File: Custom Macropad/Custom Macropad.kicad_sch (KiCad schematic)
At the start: 25 parts, among them SW1 RotaryEncoder_Switch, SW10 SW_Push, SW11 SW_Push, SW12 SW_Push, SW17 RotaryEncoder_Switch, SW2 SW_Push, SW3 SW_Push, SW5 SW_Push, SW6 SW_Push, SW7 SW_Push, SW8 SW_Push, SW9 SW_Push, U1 MOUDLE-SEEEDUINO-XIAO

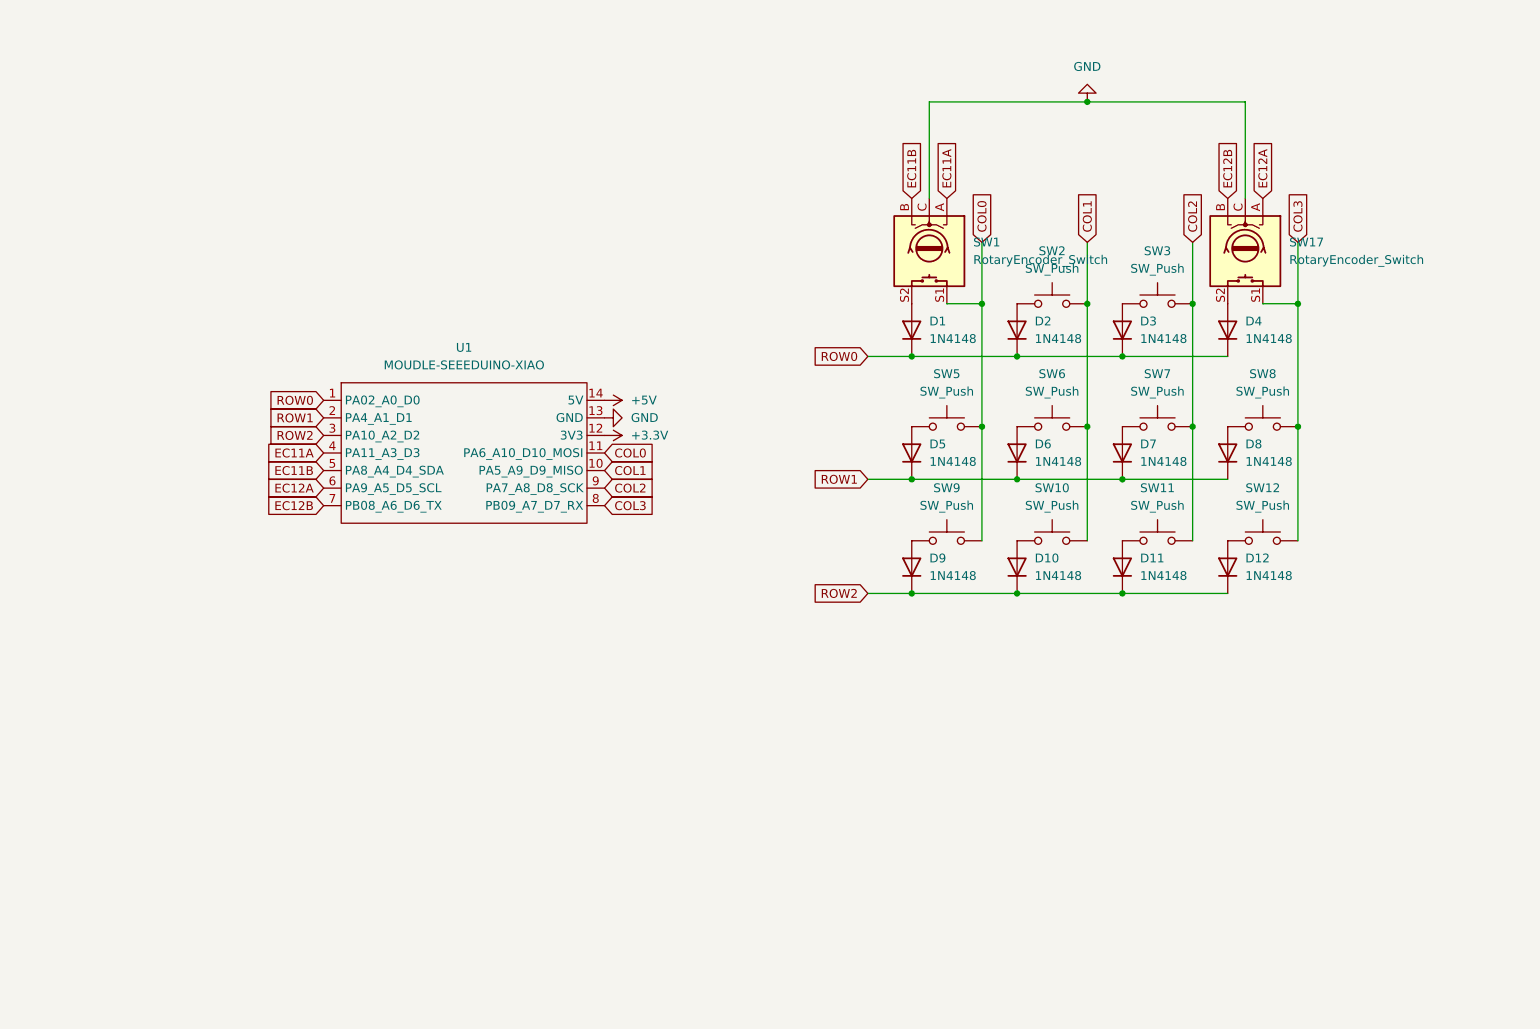
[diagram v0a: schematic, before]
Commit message: Schematic V1
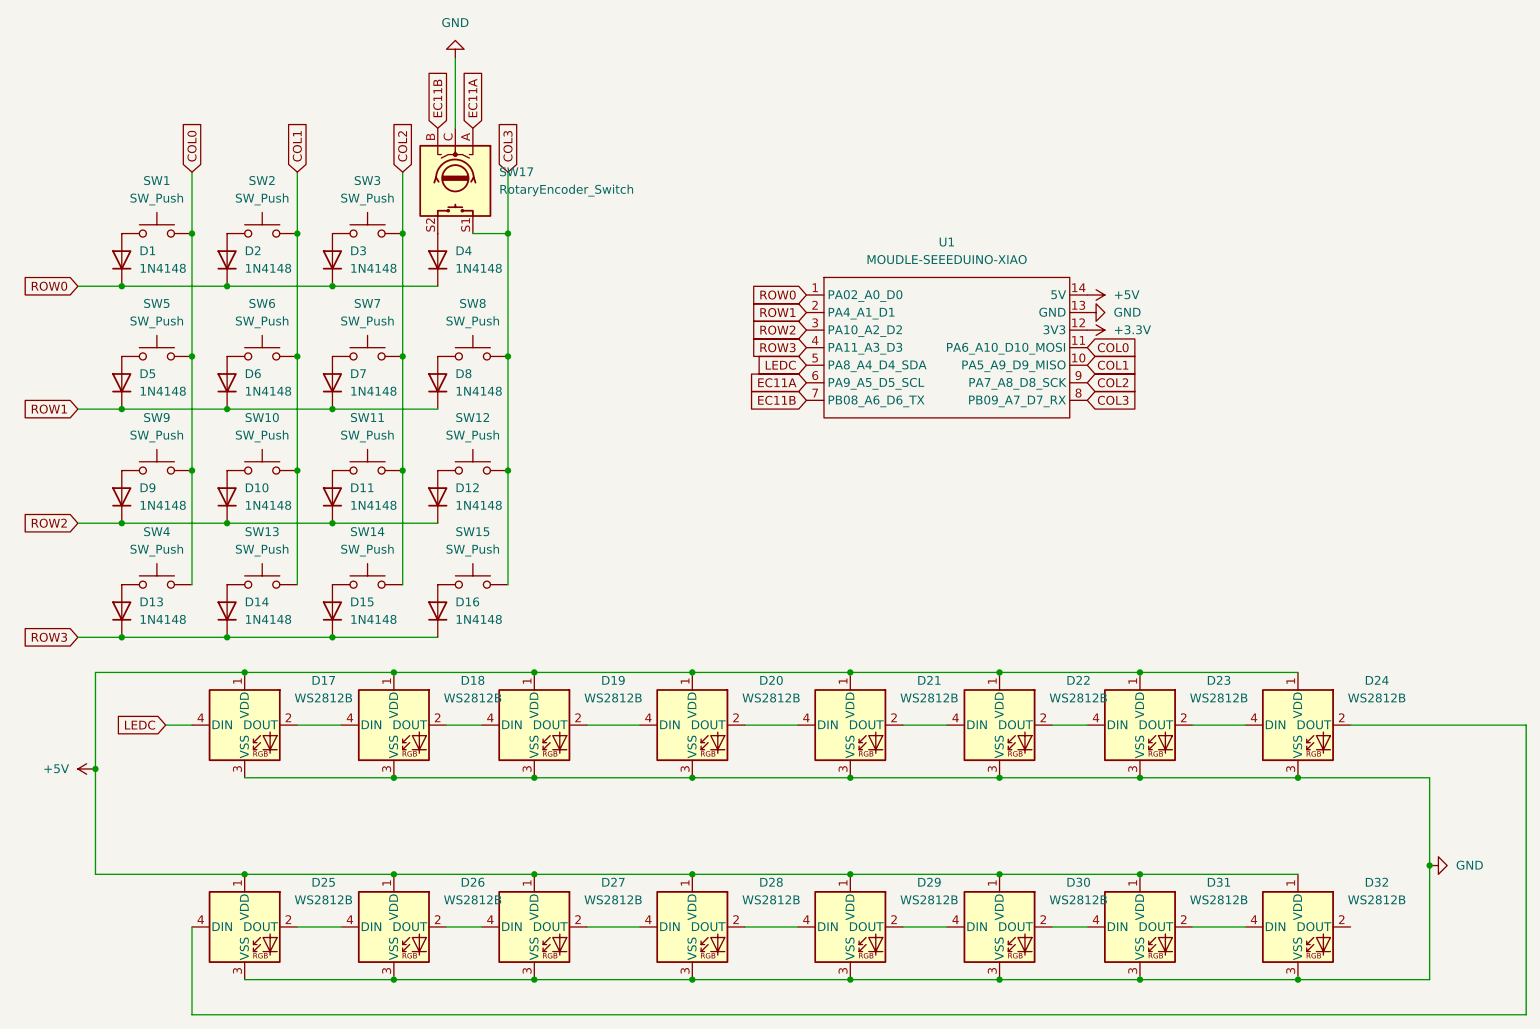
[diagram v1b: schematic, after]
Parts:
- removed SW1: RotaryEncoder_Switch, symbol Device:RotaryEncoder_Switch
- added D13, D14, D15, D16: 1N4148, Diode_THT:D_DO-35_SOD27_P7.62mm_Horizontal, symbol Diode:1N4148
- added D17, D18, D19, D20, D21, D22, D23, D24, D25, D26, D27, D28, D29, D30, D31, D32: WS2812B, LED_SMD:LED_WS2812B_PLCC4_5.0x5.0mm_P3.2mm, symbol LED:WS2812B
- added SW1, SW13, SW14, SW15, SW4: SW_Push, symbol Switch:SW_Push
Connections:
- net EC12A is gone; now on net EC11A: SW17.A, U1.6 (PA9_A5_D5_SCL)
- net EC12B is gone; now on net EC11B: SW17.B, U1.7 (PB08_A6_D6_TX)
- net +5V: now also D17.1 (VDD), D18.1 (VDD), D19.1 (VDD), D20.1 (VDD), D21.1 (VDD), D22.1 (VDD), D23.1 (VDD), D24.1 (VDD), D25.1 (VDD), D26.1 (VDD), D27.1 (VDD), D28.1 (VDD), D29.1 (VDD), D30.1 (VDD), D31.1 (VDD), D32.1 (VDD)
- net COL0: now also SW1.2, SW4.2
- net COL1: now also SW13.2
- net COL2: now also SW14.2
- net COL3: now also SW15.2
- net EC11A: no longer U1.4 (PA11_A3_D3)
- net EC11B: no longer U1.5 (PA8_A4_D4_SDA)
- net GND: now also D17.3 (VSS), D18.3 (VSS), D19.3 (VSS), D20.3 (VSS), D21.3 (VSS), D22.3 (VSS), D23.3 (VSS), D24.3 (VSS), D25.3 (VSS), D26.3 (VSS), D27.3 (VSS), D28.3 (VSS), D29.3 (VSS), D30.3 (VSS), D31.3 (VSS), D32.3 (VSS)
- net at D1.2 (A): now also SW1.1
- new net: D25.2 (DOUT), D26.4 (DIN)
- new net: D24.2 (DOUT), D25.4 (DIN)
- new net: D15.2 (A), SW14.1
- new net: D13.2 (A), SW4.1
- new net: D31.2 (DOUT), D32.4 (DIN)
- new net: D30.2 (DOUT), D31.4 (DIN)
- new net: D20.2 (DOUT), D21.4 (DIN)
- new net: D19.2 (DOUT), D20.4 (DIN)
- new net: D26.2 (DOUT), D27.4 (DIN)
- new net: D16.2 (A), SW15.1
- new net: D22.2 (DOUT), D23.4 (DIN)
- new net: D21.2 (DOUT), D22.4 (DIN)
- new net: D29.2 (DOUT), D30.4 (DIN)
- new net: D28.2 (DOUT), D29.4 (DIN)
- new net: D18.2 (DOUT), D19.4 (DIN)
- new net: D17.2 (DOUT), D18.4 (DIN)
- new net: D23.2 (DOUT), D24.4 (DIN)
- new net: D27.2 (DOUT), D28.4 (DIN)
- new net: D14.2 (A), SW13.1
- new net LEDC: D17.4 (DIN), U1.5 (PA8_A4_D4_SDA)
- new net ROW3: D13.1 (K), D14.1 (K), D15.1 (K), D16.1 (K), U1.4 (PA11_A3_D3)
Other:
- moved on the sheet: D1, D10, D11, D12, D2, D3, D4, D5, D6, D7, D8, D9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
